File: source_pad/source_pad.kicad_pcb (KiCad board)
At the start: 2 copper layers, 61.9 x 61.9 mm, 24 parts, among them SW1 SW_PUSH, SW2 SW_PUSH, SW3 SW_PUSH, SW4 SW_PUSH, SW5 SW_PUSH, SW6 SW_PUSH, SW7 SW_PUSH, SW8 SW_PUSH, SW9 SW_PUSH, U1 ProMicro-kbd

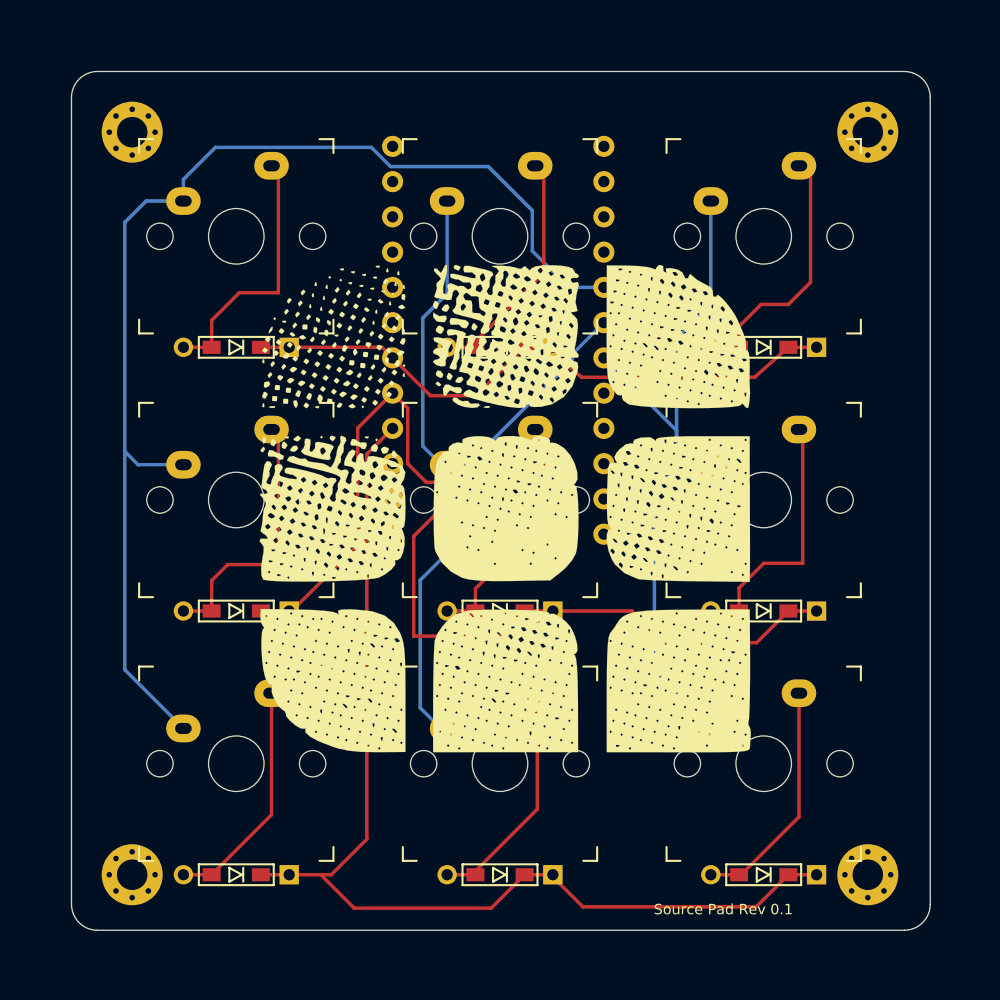
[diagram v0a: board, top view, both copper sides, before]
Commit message: Updated clearances
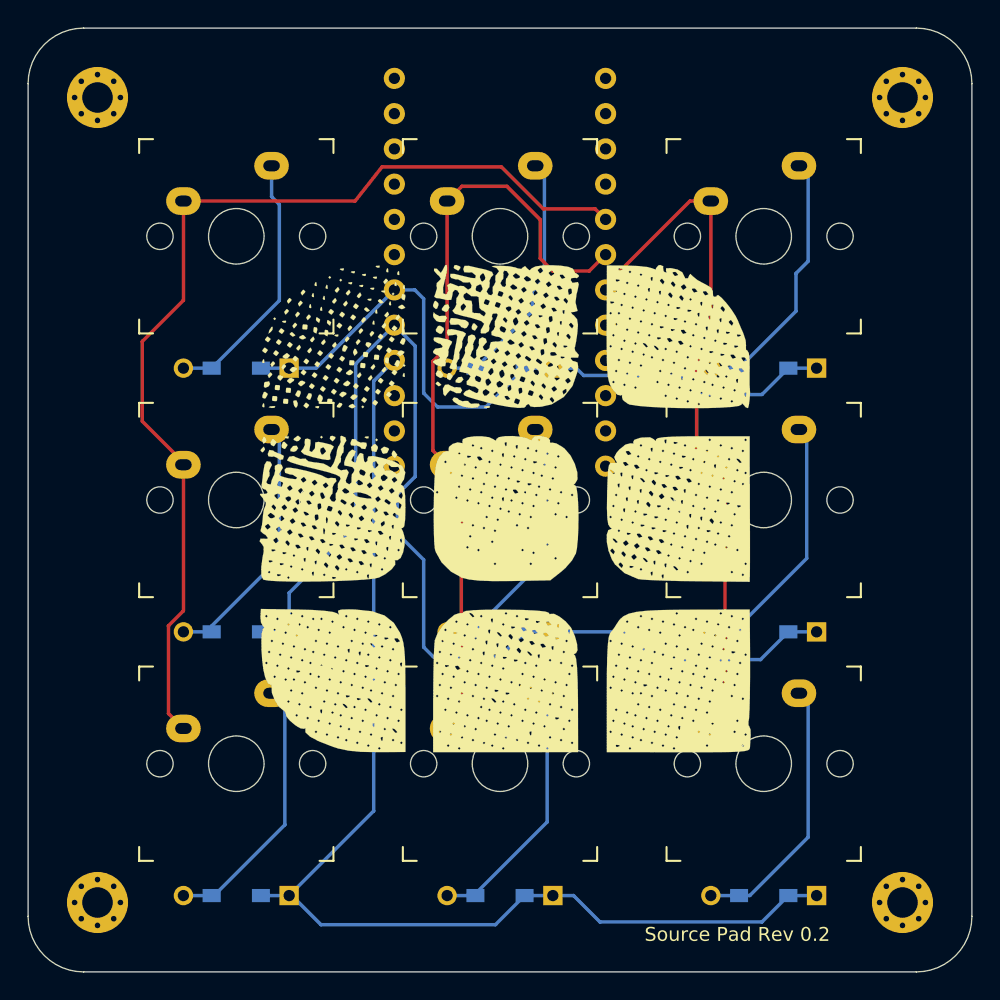
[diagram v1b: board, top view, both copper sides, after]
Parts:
- D1, D2, D3, D4, D5, D6, D7, D8, D9: moved to B.Cu
- U1: footprint kbd:ProMicro_v3.5 -> kbd:ProMicro_v3.5_fix
- moved U1 4.90 mm to (119.0, 103.1)
- moved REF** 3.54 mm to (148.0, 90.0)
- moved REF** 3.54 mm to (90.0, 90.0)
- moved REF** 3.20 mm to (90.0, 148.0)
- moved REF** 3.20 mm to (148.0, 148.0)
- moved D1 1.50 mm to (100.0, 109.5)
- moved D2 1.50 mm to (100.0, 128.5)
- moved D3 1.50 mm to (100.0, 147.5)
- moved D4 1.50 mm to (119.0, 109.5)
- moved D5 1.50 mm to (119.0, 128.5)
- moved D6 1.50 mm to (119.0, 147.5)
- moved D7 1.50 mm to (138.0, 109.5)
- moved D8 1.50 mm to (138.0, 128.5)
- moved D9 1.50 mm to (138.0, 147.5)
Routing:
- net col0: track 86.4 -> 74.6 mm
- net row1: track 74.9 -> 83.7 mm
- net row0: track 44.8 -> 52.6 mm
- net row2: track 78.9 -> 85.0 mm
- net col2: track 53.8 -> 50.1 mm
- net Net-(D9-Pad2): track 17.0 -> 19.5 mm
- net Net-(D3-Pad2): track 16.9 -> 19.3 mm
- net Net-(D4-Pad2): track 17.4 -> 18.9 mm
- net Net-(D6-Pad2): track 17.6 -> 19.1 mm
- net col1: track 57.5 -> 56.7 mm
- net Net-(D2-Pad2): track 19.5 -> 18.9 mm
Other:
- board size 61.9 x 61.9 mm -> 68 x 68 mm
- board text added: "Source Pad Rev 0.2"
- board text removed: "Source Pad Rev 0.1"
